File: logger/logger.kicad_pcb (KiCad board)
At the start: 2 copper layers, 74.2 x 69.4 mm, 88 parts, among them IC1 W25Q128JVSIQTR, IC2 TJA1050T, IC3 BNO085, J1 RJ45_Shielded, J10 Conn_01x06, J2 電源入力, J3 Conn_01x04, J4 USB_B_Micro, J6 Conn_01x02, J7 DM3AT-SF-PEJM5_40_, J8 Conn_01x03, J9 Conn_01x04, SW1 SW_Push, SW2 SW_Push, U1 NCP1117-5.0_SOT223, U2 NCP1117-3.3_SOT223, U3 RP2350_60QFN, U4 MCP2515-xSO, U5 BMP581, U6 BME280, Y1 ABM8-272-T3, Y2 ABLS-8.000MHZ-12-B-4-Y-T, Y3 NX3215SA-32.768K-STD-MUA-8

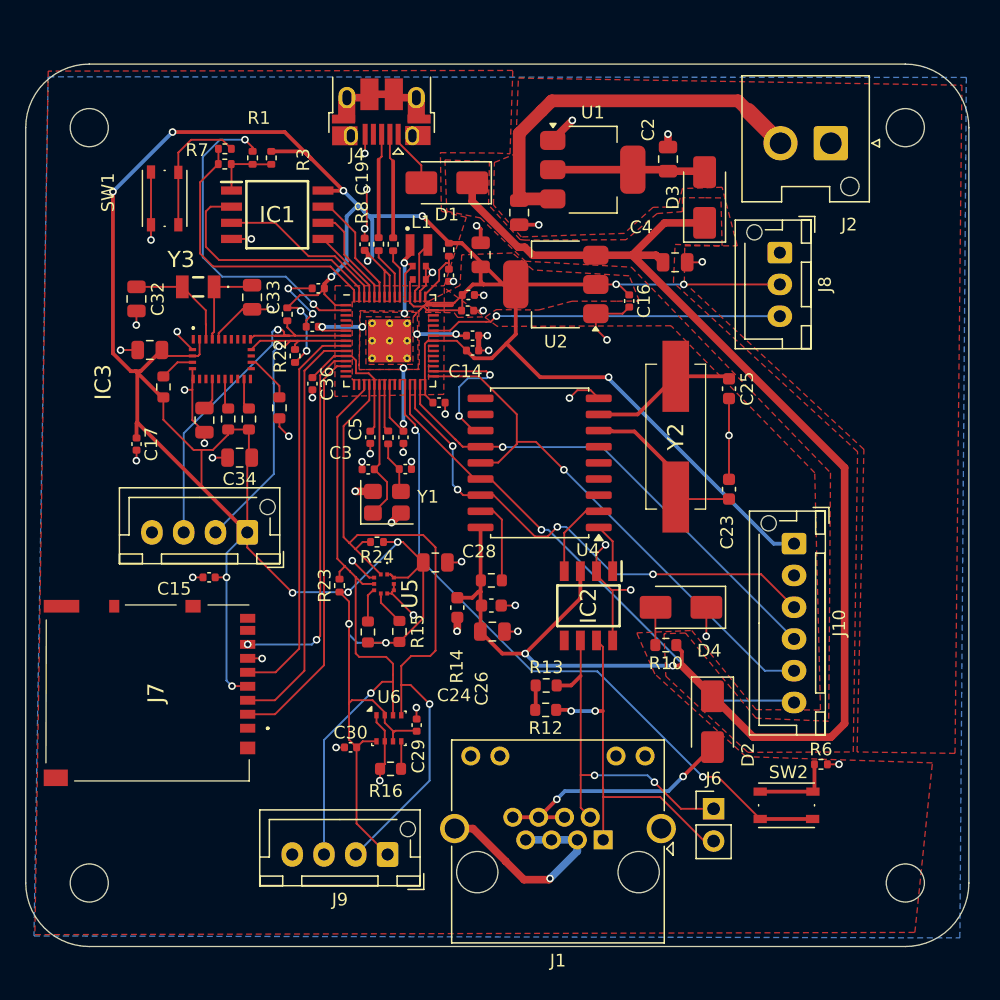
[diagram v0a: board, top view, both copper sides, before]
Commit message: 20261001
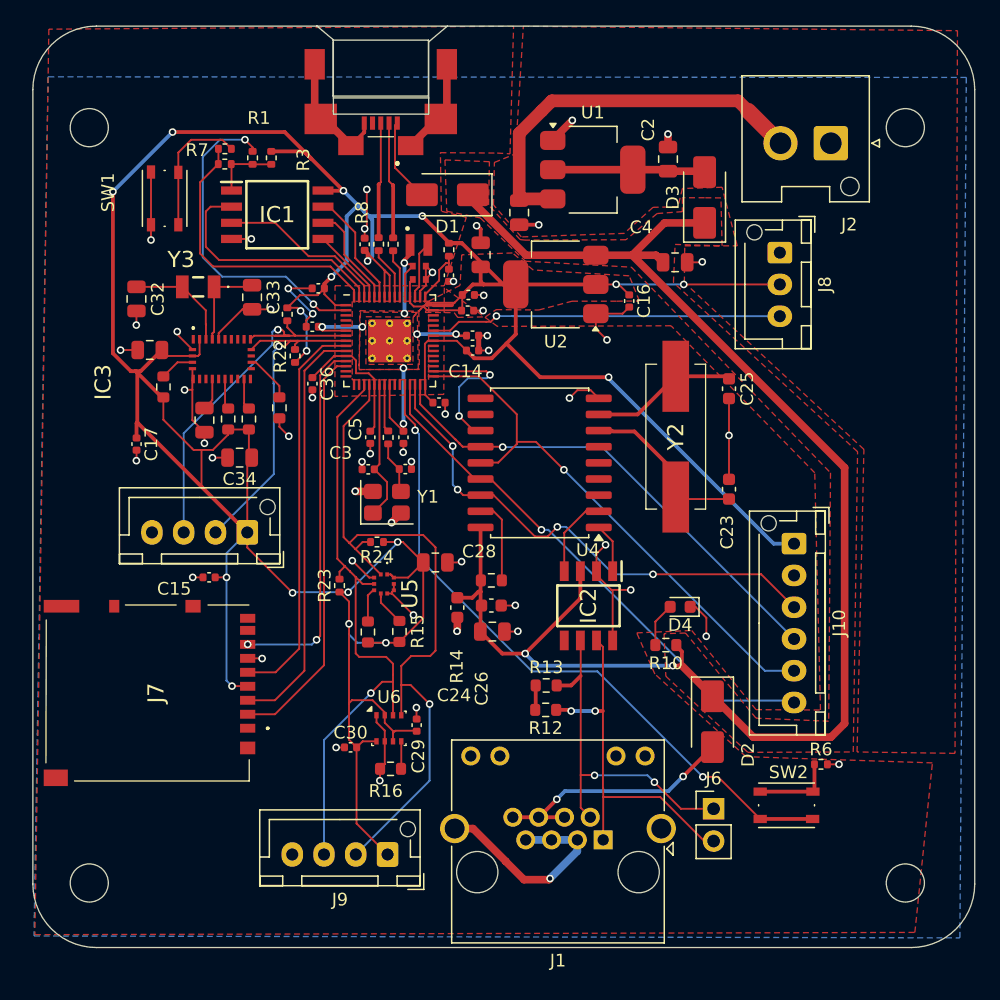
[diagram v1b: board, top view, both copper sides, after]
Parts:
- removed J4: USB_B_Micro, Connector_USB:USB_Micro-B_Amphenol_10103594-0001LF_Horizontal
- added J5: ZX62M-B-5P, footprint:ZX62MB5P, F.Cu at (110.4, 66.9)
- D4: footprint Diode_SMD:D_SMA -> LED_SMD:LED_0603_1608Metric
- moved D1 0.94 mm to (115.6, 77.2)
- moved D4 0.07 mm to (133.9, 109.6)
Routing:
- net GND: track 131.1 -> 142.4 mm, vias 54 -> 53
- net Net-(D1-A): track 4.57 -> 6.59 mm
- net +5V: track 122.0 -> 121.0 mm
- net /rp2350a/USB_D-: track 8.25 -> 9.16 mm
- net /rp2350a/USB_D+: track 8.23 -> 9.09 mm
- net Net-(D4-A): track 2.98 -> 3.49 mm
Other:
- board size 74.2 x 69.4 mm -> 74.1 x 72.5 mm
